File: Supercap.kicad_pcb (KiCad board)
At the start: 4 copper layers, 151.8 x 70 mm, 69 parts, among them IC1 NCP5109ADR2G, IC2 NCP5109ADR2G, J1 XT30, J2 XT30, J2-J1 Conn_01x10, J3 Conn_01x01, J3-J1 Conn_01x10, J4 Conn_01x01, P7803B-1000R1 P7803B-1000, P7812B-1000R1 490-P7812B-1000, U1 TLV2372, U2 TLV2372, U4 ACS71240KEXBLT-010B3, U6 LP-MSPM0G3507

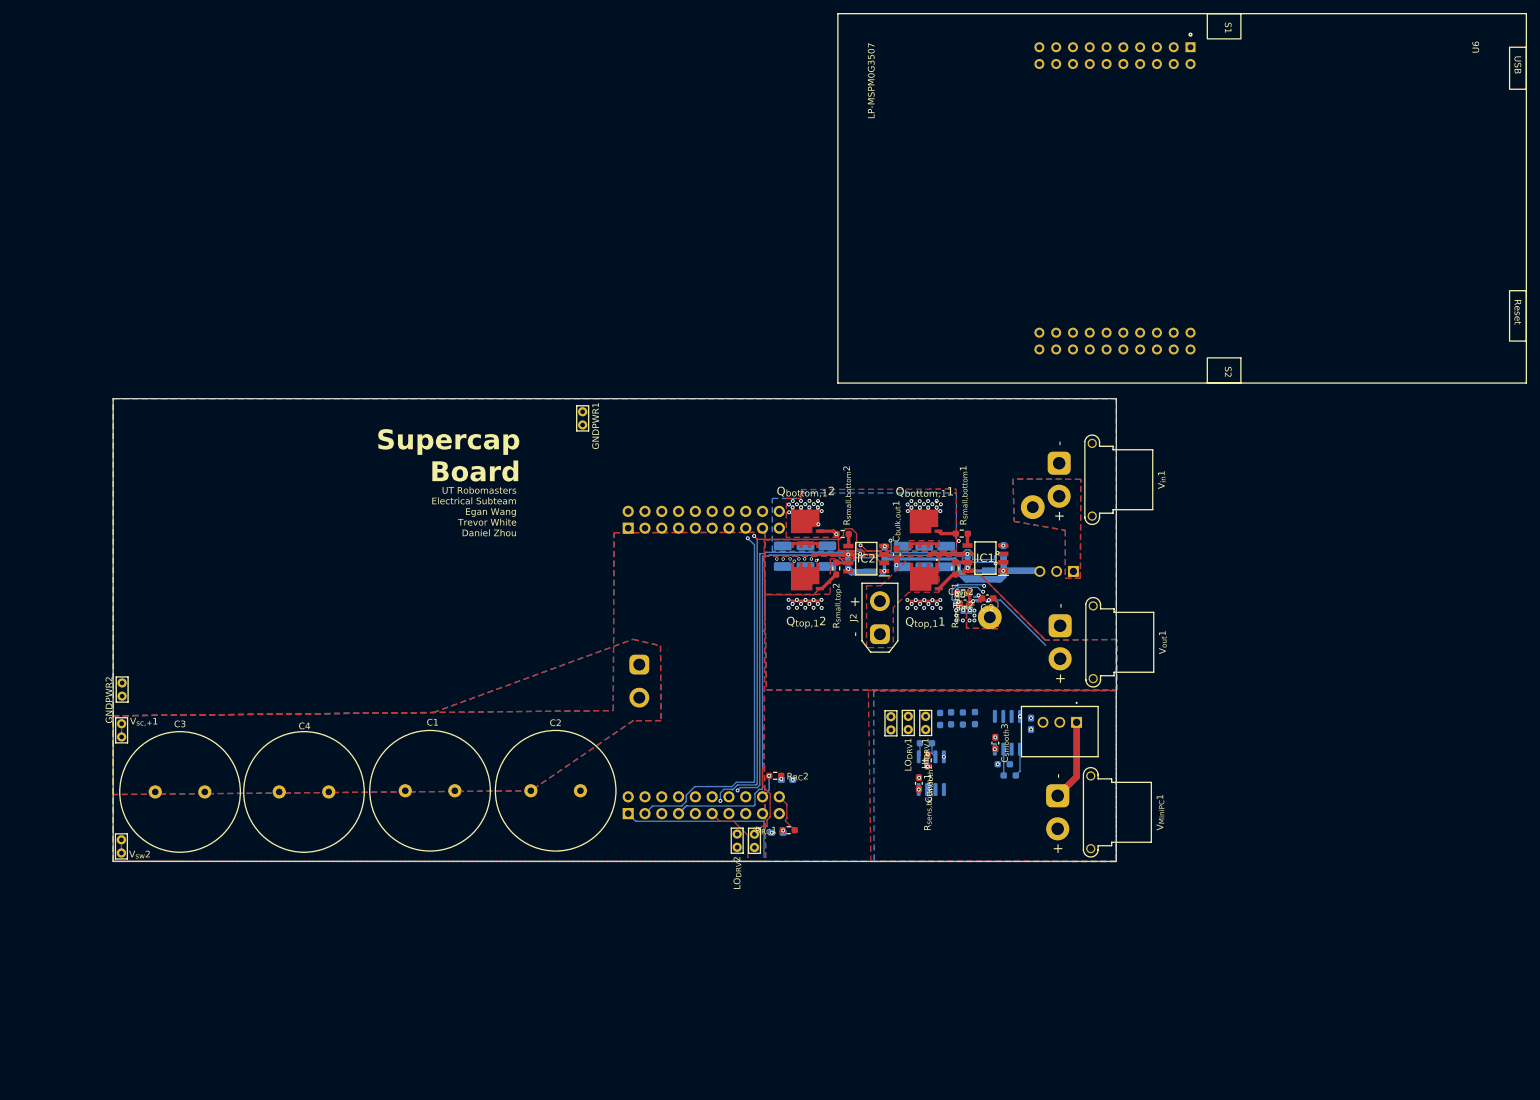
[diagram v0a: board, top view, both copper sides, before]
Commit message: laid out PCB rev C
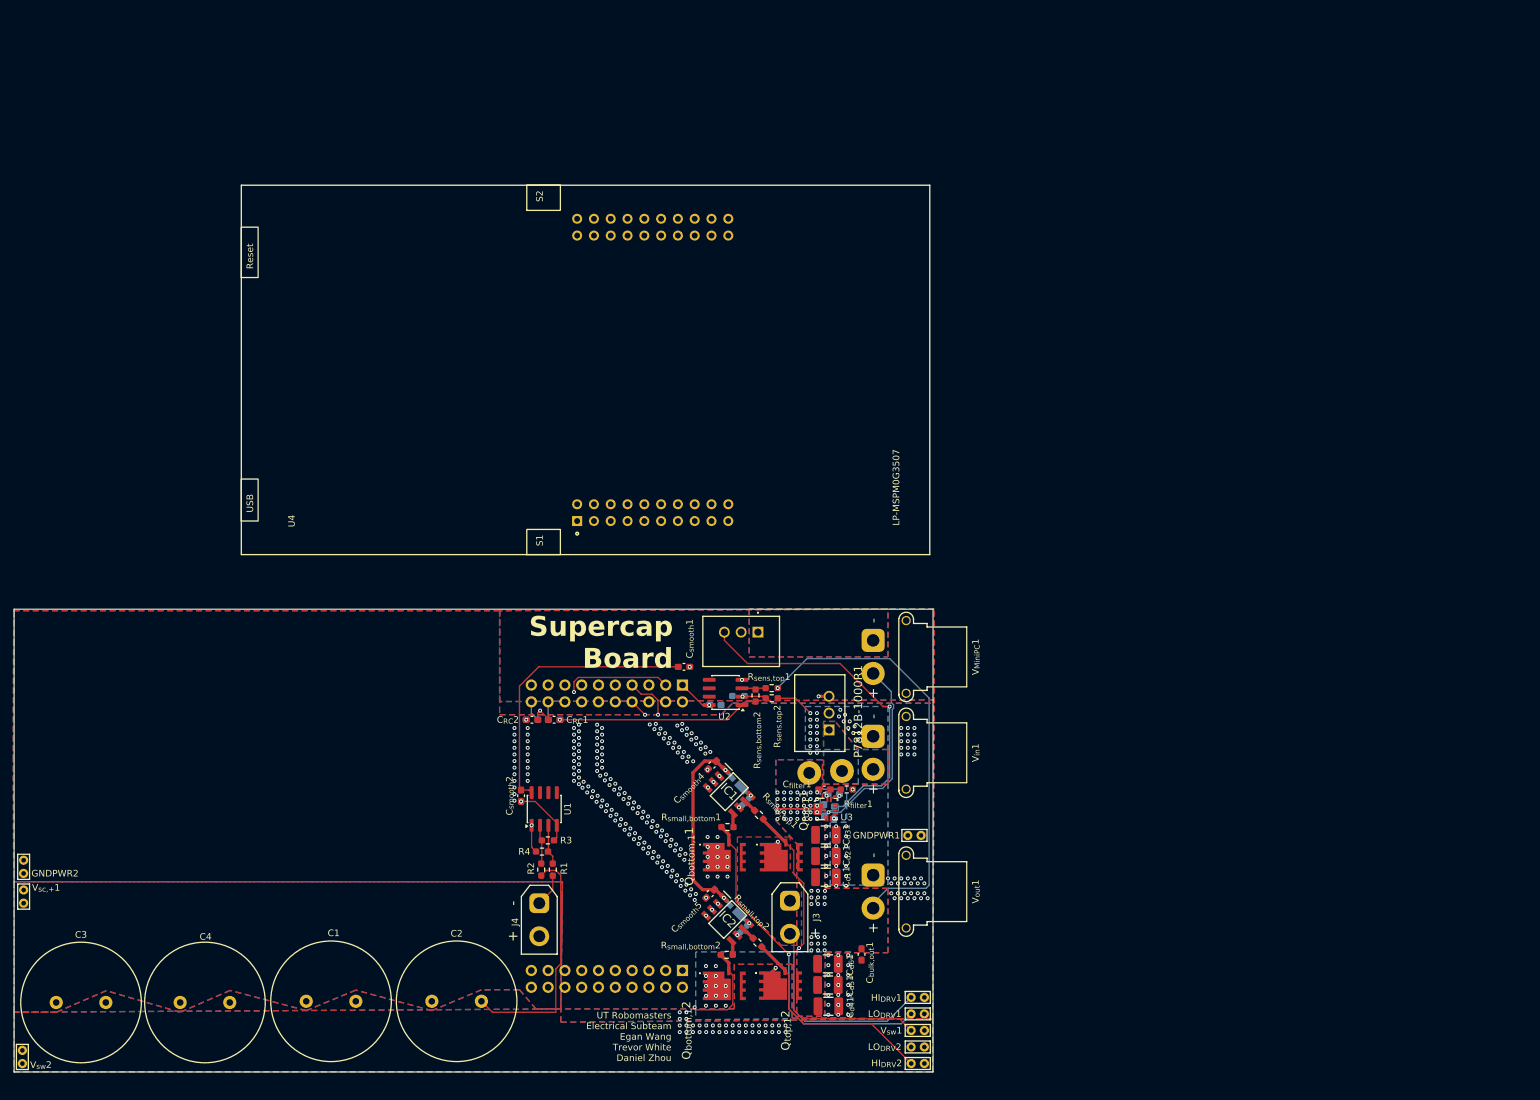
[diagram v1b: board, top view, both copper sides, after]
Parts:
- added C_{filter}1: 10u, Capacitor_SMD:C_0603_1608Metric_Pad1.08x0.95mm_HandSolder, F.Cu at (145.2, 130.4)
- added R_{filter}1: 3.3, Resistor_SMD:R_0603_1608Metric_Pad0.98x0.95mm_HandSolder, F.Cu at (148.5, 130.4)
- C_{RC}1: renamed from C_{RC}2; moved to F.Cu
- C_{RC}2: renamed from C_{RC}1; moved to F.Cu
- C_{byp}1: renamed from C_{byp}2; moved to B.Cu
- C_{d1}1, C_{d2}1, C_{d3}1, C_{d4}1, C_{d5}1, C_{d6}1, P7812B-1000R1, R1, R2, R3, R4, R_{sens,bottom}2, R_{sens,top}1, R_{sens,top}2, U1, U2: moved to F.Cu
- C_{l}1: renamed from C_{l}2; moved to B.Cu
- C_{smooth}2: renamed from C_{smooth}1; moved to F.Cu
- C_{smooth}3: renamed from C_{smooth}2; moved to B.Cu
- C_{smooth}4: renamed from C_{smooth}6; moved to F.Cu
- C_{smooth}5: renamed from C_{smooth}7; moved to F.Cu
- J2: renamed from J4; moved to B.Cu
- J4: renamed from J1; moved to F.Cu
- R_{RC}1: renamed from R_{RC}2; moved to B.Cu
- R_{RC}2: renamed from R_{RC}1; moved to B.Cu
- R_{pu}1: renamed from R_{pu}2; moved to B.Cu
- R_{sens,bottom}1: moved to B.Cu
- U3: renamed from U4; moved to F.Cu
- moved U4 91.5 mm to (110.3, 66.9), turned to 90 degrees
- moved GNDPWR1 79.2 mm to (157.8, 137.3), turned to 0 degrees
- moved C_{smooth}2 77.9 mm to (99.3, 131.3)
- moved R4 71.7 mm to (102.4, 139.8), turned to 180 degrees
- moved U1 71.0 mm to (102.8, 133.3)
- moved Q_{bottom,1}2 70.4 mm to (130.1, 160.0), turned to -90 degrees
- moved R3 69.9 mm to (103.3, 138.1), turned to 0 degrees
- moved C_{d4}1 68.1 mm to (145.7, 163.2), turned to 0 degrees
- moved J2-J1 67.4 mm to (123.7, 157.8), turned to 90 degrees
- moved R_{small,bottom}2 66.0 mm to (130.4, 155.4)
- moved C_{d5}1 65.0 mm to (145.7, 160.0), turned to 0 degrees
- moved R2 64.5 mm to (102.3, 142.5), turned to 90 degrees
- moved R1 64.4 mm to (104.1, 142.5), turned to 90 degrees
- moved C_{d6}1 62.7 mm to (145.7, 156.8), turned to 0 degrees
- moved C_{bulk,out}1 60.7 mm to (150.8, 155.3), turned to -90 degrees
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- renumbered C_{smooth}3 to C_{smooth}1, J3 to J1, J2 to J3, U6 to U4
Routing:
- net /Control/PA22: track 92.8 -> 18.1 mm, vias 4 -> 2
- net /Control/PA8: track 92.1 -> 20.2 mm, vias 1 -> 2
- net /Control/I_{bat,out+}: track 0.00 -> 65.9 mm, vias 34 -> 33
- net /Control/+3V3: track 42.9 -> 100.1 mm, vias 6 -> 3
- net /Control/F_bat: track 25.3 -> 74.5 mm, vias 2 -> 1
- net /Voltage Converter/V_{sw,2}: track 7.37 -> 48.1 mm, vias 9 -> 40
- net /Control/I_bat: track 28.0 -> 66.8 mm
- net /Control/PB9: track 72.6 -> 41.6 mm, vias 2 -> 1
- net /Voltage Converter/HI_DRV_{1}: track 23.1 -> 54.0 mm, vias 0 -> 1
- net /Control/V_{bat,sens}: track 2.09 -> 30.7 mm
- net /Housekeeping/+12V: track 32.0 -> 55.9 mm, vias 2 -> 3
- net /Control/PA25: track 80.3 -> 57.8 mm
- net /Voltage Converter/V_{sw,1}: track 25.7 -> 44.4 mm, vias 1 -> 2
- net /Voltage Converter/LO_DRV_{1}: track 36.0 -> 53.8 mm
- net /Control/V_{sc,sens}: track 4.24 -> 21.1 mm, vias 1 -> 2
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- added copper zone on B.Cu, net /Control/+3V3
- added copper zone on B.Cu, net /Housekeeping/MiniPC
- added copper zone on F.Cu, net /Housekeeping/MiniPC
- added copper zone on In1.Cu, net /Housekeeping/MiniPC
- added copper zone on In2.Cu, net /Housekeeping/MiniPC
- added copper zone on In1.Cu, net GND
- removed copper zone on In1.Cu, net /Control/+3V3
- removed copper zone on In1.Cu, net /Voltage Converter/V_{sw,1}
- removed copper zone on In2.Cu, net /Voltage Converter/V_{sw,1}
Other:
- board size 151.8 x 70 mm -> 139 x 70 mm
- board text added: "Power Inductor Size"
